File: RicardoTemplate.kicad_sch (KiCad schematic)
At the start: 39 parts, among them J1 RBUS, U1 ESP32-S3, Y1 R940000171

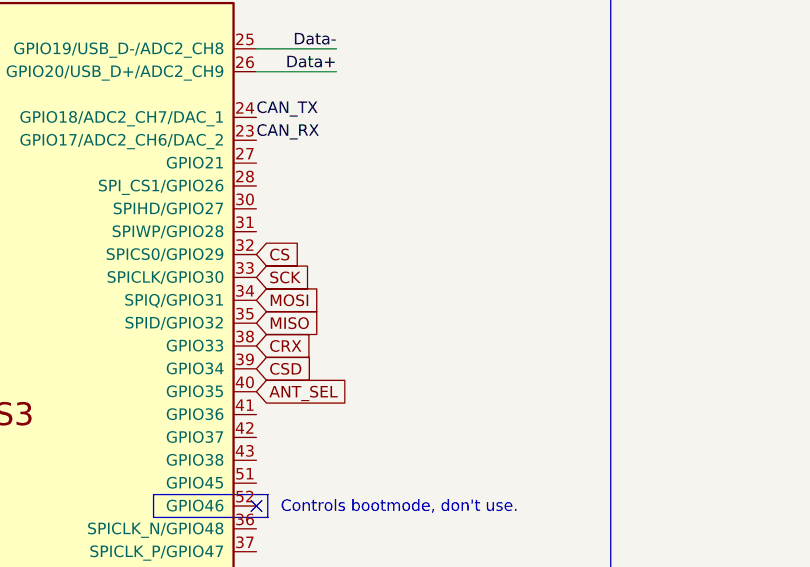
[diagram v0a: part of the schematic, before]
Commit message: Minor improvements
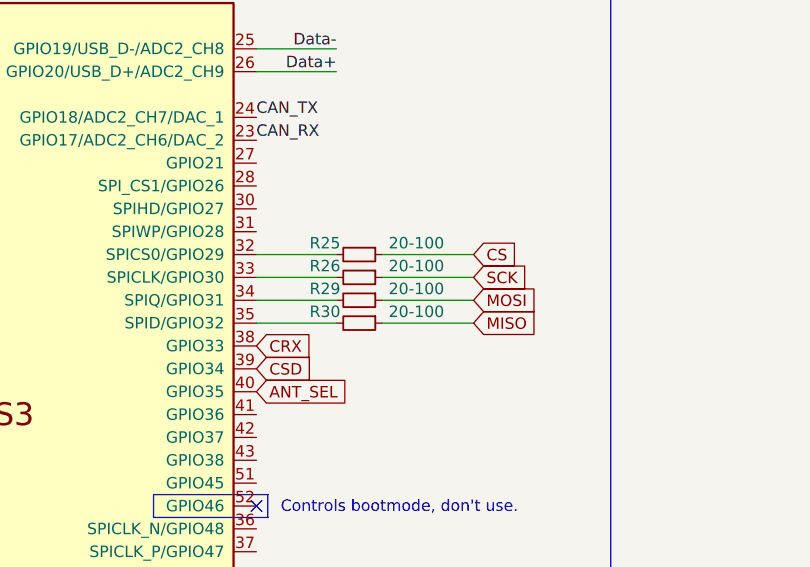
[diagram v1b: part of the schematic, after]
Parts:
- added R25, R26, R29, R30: 20-100, Resistor_SMD:R_0402_1005Metric, symbol Device:R_Small
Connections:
- net CS: now also R25.1; no longer U1.32 (SPICS0/GPIO29)
- net MISO: now also R30.1; no longer U1.35 (SPID/GPIO32)
- net MOSI: now also R29.1; no longer U1.34 (SPIQ/GPIO31)
- net SCK: now also R26.1; no longer U1.33 (SPICLK/GPIO30)
- new net: R29.2, U1.34 (SPIQ/GPIO31)
- new net: R25.2, U1.32 (SPICS0/GPIO29)
- new net: R26.2, U1.33 (SPICLK/GPIO30)
- new net: R30.2, U1.35 (SPID/GPIO32)
